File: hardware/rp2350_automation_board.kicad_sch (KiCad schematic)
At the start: 0 parts

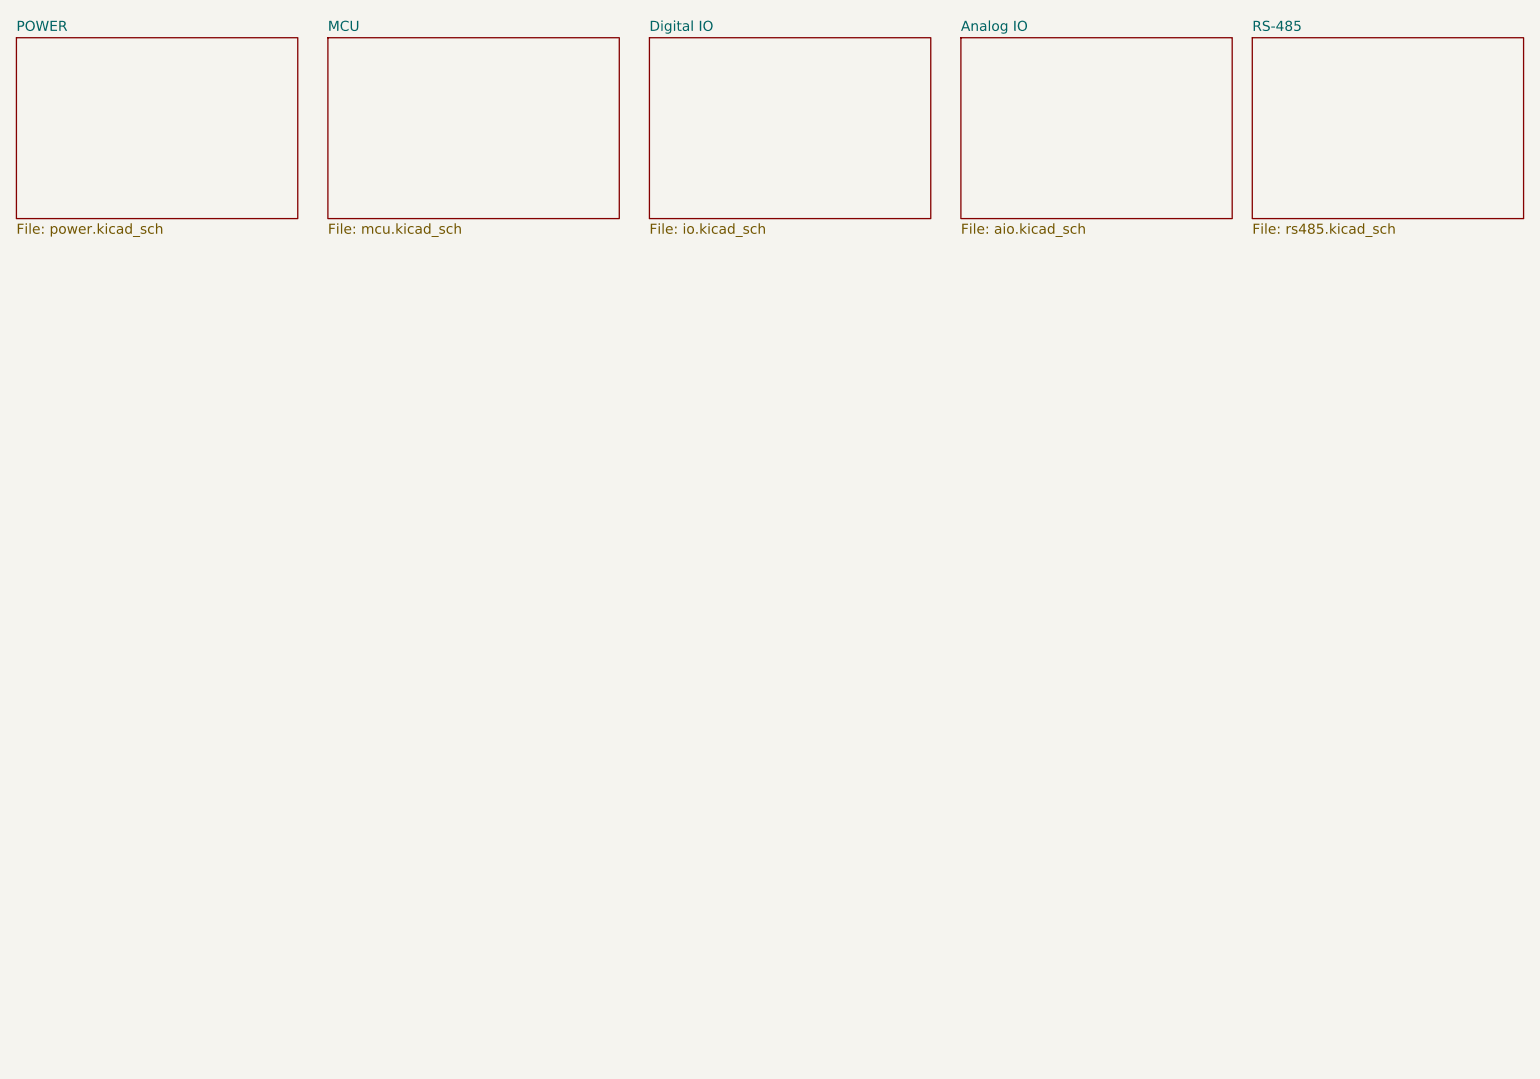
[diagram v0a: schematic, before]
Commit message: Board complete
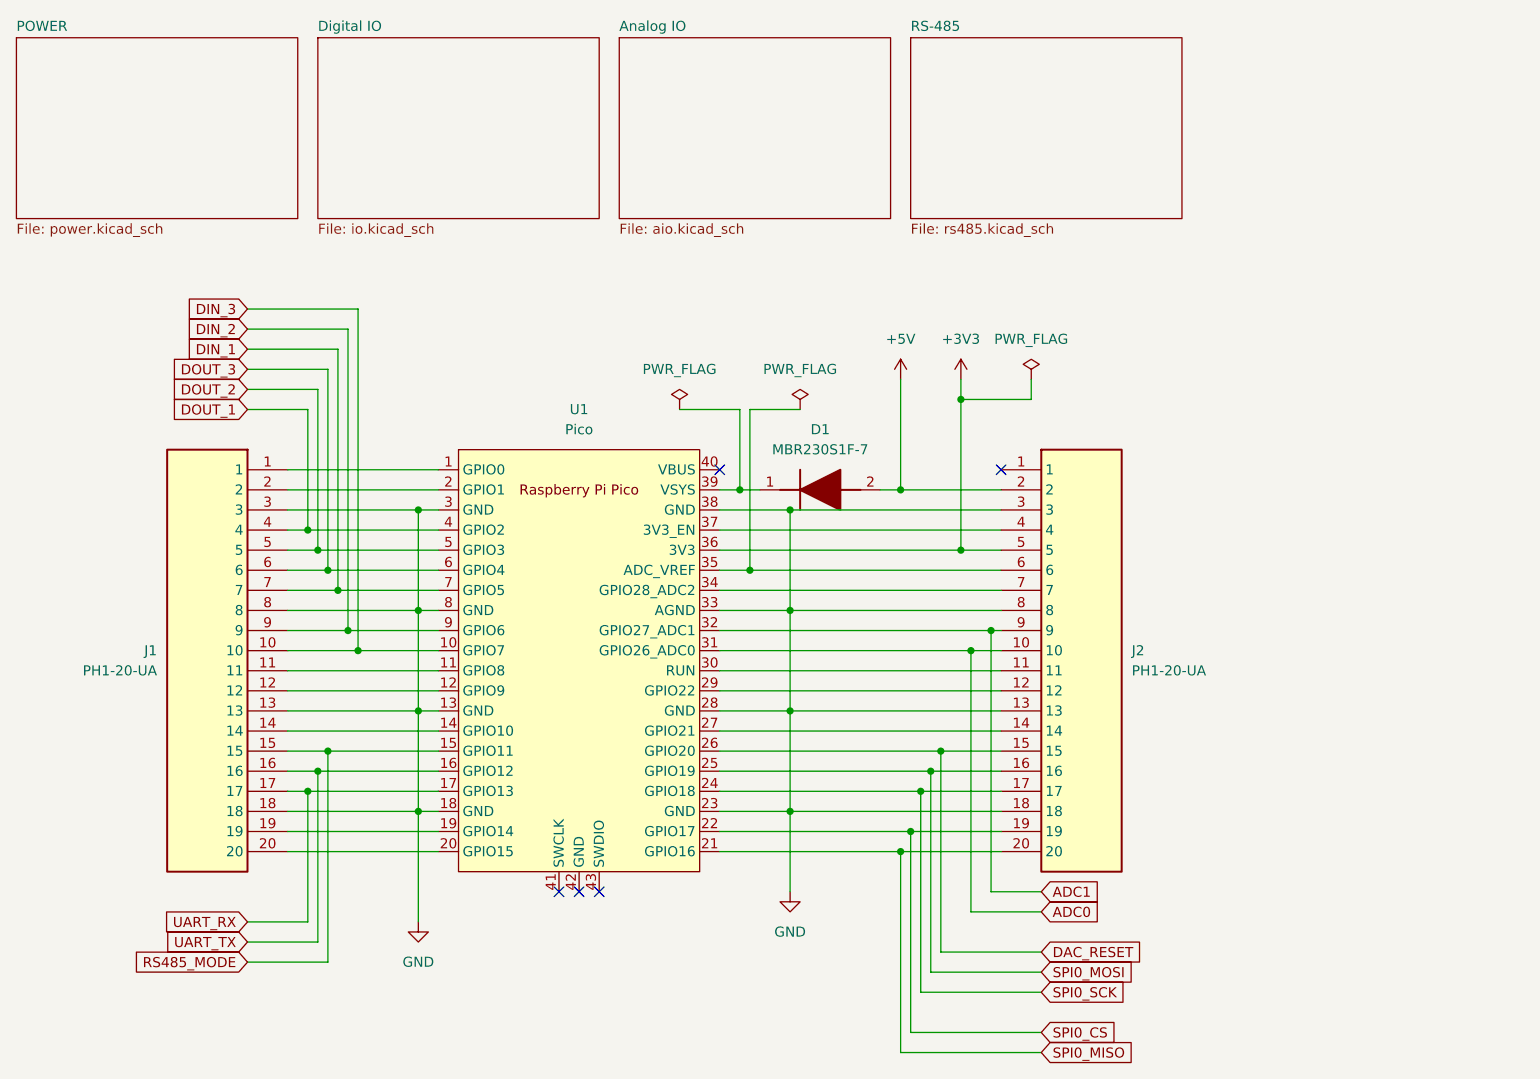
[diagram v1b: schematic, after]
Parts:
- added D1: MBR230S1F-7, Samacsys:SODFL3518X115N, symbol Samacsys:MBR230S1F-7
- added J1, J2: PH1-20-UA, Samacsys:HDRV20W64P0X254_1X20_5080X249X886P, symbol Samacsys:PH1-20-UA
- added U1: Pico, RP-Pico Libraries:RPi_Pico_SMD_TH, symbol RP_Pico:Pico
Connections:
- new net: J1.1, U1.1 (GPIO0)
- new net: J1.11, U1.11 (GPIO8)
- new net: J1.12, U1.12 (GPIO9)
- new net: J1.14, U1.14 (GPIO10)
- new net: J1.19, U1.19 (GPIO14)
- new net: J1.2, U1.2 (GPIO1)
- new net: J1.20, U1.20 (GPIO15)
- new net: J2.14, U1.27 (GPIO21)
- new net: J2.12, U1.29 (GPIO22)
- new net: J2.11, U1.30 (RUN)
- new net: J2.7, U1.34 (GPIO28_ADC2)
- new net: J2.6, U1.35 (ADC_VREF)
- new net: J2.4, U1.37 (3V3_EN)
- new net: D1.1 (K), U1.39 (VSYS)
- new net +3V3: J2.5, U1.36 (3V3)
- new net +5V: D1.2 (A), J2.2
- new net ADC0: J2.10, U1.31 (GPIO26_ADC0)
- new net ADC1: J2.9, U1.32 (GPIO27_ADC1)
- new net DAC_RESET: J2.15, U1.26 (GPIO20)
- new net DIN_1: J1.7, U1.7 (GPIO5)
- new net DIN_2: J1.9, U1.9 (GPIO6)
- new net DIN_3: J1.10, U1.10 (GPIO7)
- new net DOUT_1: J1.4, U1.4 (GPIO2)
- new net DOUT_2: J1.5, U1.5 (GPIO3)
- new net DOUT_3: J1.6, U1.6 (GPIO4)
- new net GND: J1.13, J1.18, J1.3, J1.8, J2.13, J2.18, J2.3, J2.8, U1.13 (GND), U1.18 (GND), U1.23 (GND), U1.28 (GND), U1.3 (GND), U1.33 (AGND), U1.38 (GND), U1.8 (GND)
- new net RS485_MODE: J1.15, U1.15 (GPIO11)
- new net SPI0_CS: J2.19, U1.22 (GPIO17)
- new net SPI0_MISO: J2.20, U1.21 (GPIO16)
- new net SPI0_MOSI: J2.16, U1.25 (GPIO19)
- new net SPI0_SCK: J2.17, U1.24 (GPIO18)
- new net UART_RX: J1.17, U1.17 (GPIO13)
- new net UART_TX: J1.16, U1.16 (GPIO12)
- no-connect marks 0 -> 5
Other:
- removed sheet MCU
